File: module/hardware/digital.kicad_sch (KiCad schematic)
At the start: 36 parts, among them J10 Conn_01x03, J11 Conn_01x03, J12 Conn_01x03, J5 Conn_01x03_Male, J6 Conn_01x03_Male, J7 Conn_01x03, J8 Conn_01x03, J9 Conn_01x05_Male, SW2 SW_Push, U8 W25Q128JVS, U9 RP2040, Y1 12MHz 18pF

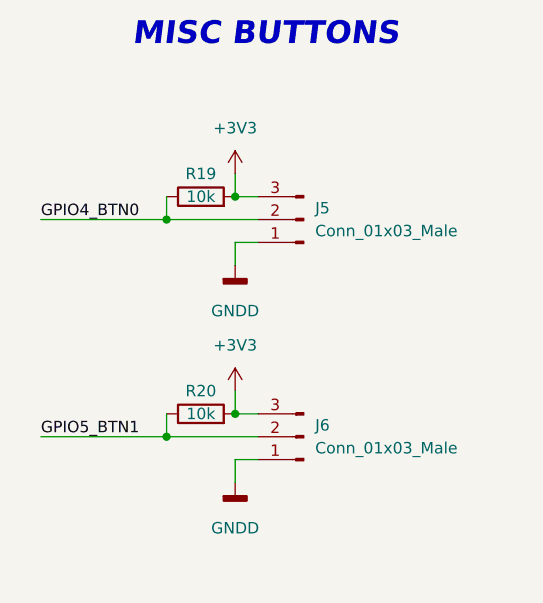
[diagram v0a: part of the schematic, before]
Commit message: Route/move USB
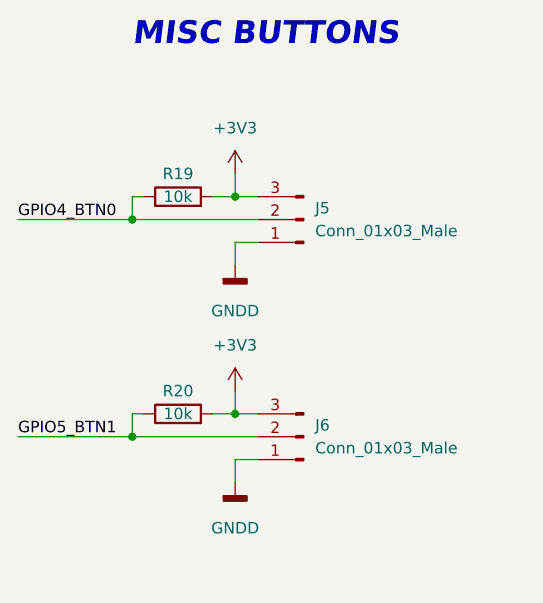
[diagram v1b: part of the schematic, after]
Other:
- moved on the sheet: R19, R20
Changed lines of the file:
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@@
   (junction (at 318.77 40.64) (diameter 0) (color 0 0 0 0)
   )
+  (junction (at 58.42 86.36) (diameter 0) (color 0 0 0 0)
+  )
   (junction (at 240.03 143.51) (diameter 0) (color 0 0 0 0)
   )
@@
   (junction (at 92.71 213.36) (diameter 0) (color 0 0 0 0)
   )
+  (junction (at 58.42 62.23) (diameter 0) (color 0 0 0 0)
+  )
   (junction (at 242.57 55.88) (diameter 0) (color 0 0 0 0)
   )
@@
   (junction (at 295.91 40.64) (diameter 0) (color 0 0 0 0)
   )
-  (junction (at 62.23 62.23) (diameter 0) (color 0 0 0 0)
-  )
   (junction (at 341.63 54.61) (diameter 0) (color 0 0 0 0)
   )
@@
   )
   (junction (at 78.74 144.78) (diameter 0) (color 0 0 0 0)
-  )
-  (junction (at 62.23 86.36) (diameter 0) (color 0 0 0 0)
   )
   (junction (at 231.14 40.64) (diameter 0) (color 0 0 0 0)
@@
     (stroke (width 0) (type default) (color 0 0 0 0))
   )
-  (wire (pts (xy 62.23 59.69) (xy 62.23 62.23))
+  (wire (pts (xy 58.42 59.69) (xy 58.42 62.23))
     (stroke (width 0) (type default) (color 0 0 0 0))
   )
@@
     (stroke (width 0) (type default) (color 0 0 0 0))
   )
+  (wire (pts (xy 58.42 59.69) (xy 59.69 59.69))
+    (stroke (width 0) (type default) (color 0 0 0 0))
+  )
   (wire (pts (xy 114.3 128.27) (xy 127 128.27))
     (stroke (width 0) (type default) (color 0 0 0 0))
   )
+  (wire (pts (xy 58.42 86.36) (xy 72.39 86.36))
+    (stroke (width 0) (type default) (color 0 0 0 0))
+  )
   (wire (pts (xy 114.3 120.65) (xy 114.3 123.19))
     (stroke (width 0) (type default) (color 0 0 0 0))
@@
     (stroke (width 0) (type default) (color 0 0 0 0))
   )
-  (wire (pts (xy 62.23 86.36) (xy 72.39 86.36))
-    (stroke (width 0) (type default) (color 0 0 0 0))
-  )
   (wire (pts (xy 231.14 36.83) (xy 231.14 40.64))
     (stroke (width 0) (type default) (color 0 0 0 0))
@@
     (stroke (width 0) (type default) (color 0 0 0 0))
   )
-  (wire (pts (xy 62.23 83.82) (xy 62.23 86.36))
+  (wire (pts (xy 58.42 83.82) (xy 58.42 86.36))
     (stroke (width 0) (type default) (color 0 0 0 0))
   )
@@
     (stroke (width 0) (type default) (color 0 0 0 0))
   )
-  (wire (pts (xy 62.23 62.23) (xy 72.39 62.23))
+  (wire (pts (xy 58.42 62.23) (xy 72.39 62.23))
     (stroke (width 0) (type default) (color 0 0 0 0))
   )
@@
     (stroke (width 0) (type default) (color 0 0 0 0))
   )
-  (wire (pts (xy 48.26 62.23) (xy 62.23 62.23))
+  (wire (pts (xy 45.72 62.23) (xy 58.42 62.23))
     (stroke (width 0) (type default) (color 0 0 0 0))
   )
@@
     (stroke (width 0) (type default) (color 0 0 0 0))
   )
+  (wire (pts (xy 67.31 59.69) (xy 69.85 59.69))
+    (stroke (width 0) (type default) (color 0 0 0 0))
+  )
+  (wire (pts (xy 58.42 83.82) (xy 59.69 83.82))
+    (stroke (width 0) (type default) (color 0 0 0 0))
+  )
   (wire (pts (xy 240.03 143.51) (xy 240.03 153.67))
     (stroke (width 0) (type default) (color 0 0 0 0))
@@
     (stroke (width 0) (type default) (color 0 0 0 0))
   )
-  (wire (pts (xy 48.26 86.36) (xy 62.23 86.36))
+  (wire (pts (xy 45.72 86.36) (xy 58.42 86.36))
     (stroke (width 0) (type default) (color 0 0 0 0))
   )
@@
   )
   (wire (pts (xy 242.57 90.17) (xy 233.68 90.17))
+    (stroke (width 0) (type default) (color 0 0 0 0))
+  )
+  (wire (pts (xy 67.31 83.82) (xy 69.85 83.82))
     (stroke (width 0) (type default) (color 0 0 0 0))
   )
@@
     (effects (font (size 1.27 1.27)) (justify right bottom))
   )
-  (label "GPIO4_BTN0" (at 48.26 62.23 0)
+  (label "GPIO4_BTN0" (at 45.72 62.23 0)
     (effects (font (size 1.27 1.27)) (justify left bottom))
   )
@@
     (effects (font (size 1.27 1.27)) (justify left bottom))
   )
-  (label "GPIO5_BTN1" (at 48.26 86.36 0)
+  (label "GPIO5_BTN1" (at 45.72 86.36 0)
     (effects (font (size 1.27 1.27)) (justify left bottom))
   )
@@
     (pin "1")
   )
-  (symbol (lib_id "Device:R") (at 66.04 59.69 90) (unit 1)
+  (symbol (lib_id "Device:R") (at 63.5 59.69 90) (unit 1)
     (in_bom yes) (on_board yes)
-    (property "Reference" "R19" (id 0) (at 66.04 57.15 90))
-    (property "Value" "10k" (id 1) (at 66.04 59.69 90))
-    (property "Footprint" "Resistor_SMD:R_0603_1608Metric_Pad0.98x0.95mm_HandSolder" (id 2) (at 66.04 61.468 90)
-      (effects (font (size 1.27 1.27)) hide)
-    )
-    (property "Datasheet" "~" (id 3) (at 66.04 59.69 0)
+    (property "Reference" "R19" (id 0) (at 63.5 57.15 90))
+    (property "Value" "10k" (id 1) (at 63.5 59.69 90))
+    (property "Footprint" "Resistor_SMD:R_0603_1608Metric_Pad0.98x0.95mm_HandSolder" (id 2) (at 63.5 61.468 90)
+      (effects (font (size 1.27 1.27)) hide)
+    )
+    (property "Datasheet" "~" (id 3) (at 63.5 59.69 0)
       (effects (font (size 1.27 1.27)) hide)
     )
@@
     (pin "2")
   )
-  (symbol (lib_id "Device:R") (at 66.04 83.82 90) (unit 1)
+  (symbol (lib_id "Device:R") (at 63.5 83.82 90) (unit 1)
     (in_bom yes) (on_board yes)
-    (property "Reference" "R20" (id 0) (at 66.04 81.28 90))
-    (property "Value" "10k" (id 1) (at 66.04 83.82 90))
-    (property "Footprint" "Resistor_SMD:R_0603_1608Metric_Pad0.98x0.95mm_HandSolder" (id 2) (at 66.04 85.598 90)
-      (effects (font (size 1.27 1.27)) hide)
-    )
-    (property "Datasheet" "~" (id 3) (at 66.04 83.82 0)
-      (effects (font (size 1.27 1.27)) hide)
-    )
+    (property "Reference" "R20" (id 0) (at 63.5 81.28 90))
+    (property "Value" "10k" (id 1) (at 63.5 83.82 90))
+    (property "Footprint" "Resistor_SMD:R_0603_1608Metric_Pad0.98x0.95mm_HandSolder" (id 2) (at 63.5 85.598 90)
+      (effects (font (size 1.27 1.27)) hide)
+    )
+    (property "Datasheet" "~" (id 3) (at 63.5 83.82 0)
+      (effects (font (size 1.27 1.27)) hide)
+    )
